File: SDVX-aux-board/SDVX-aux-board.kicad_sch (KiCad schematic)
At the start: 6 parts, among them CN1 AudioJack4_SwitchTR1, CN2 Conn_01x04

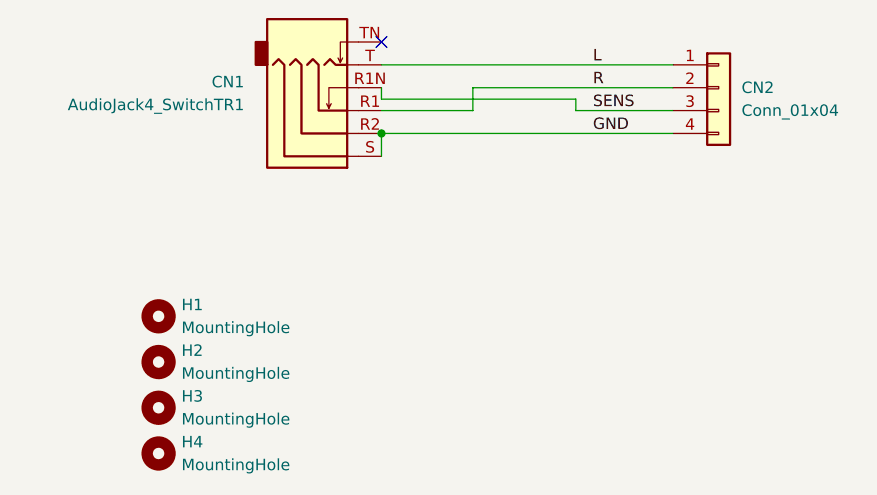
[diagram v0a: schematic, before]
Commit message: Update to working design (kicad 8.0)
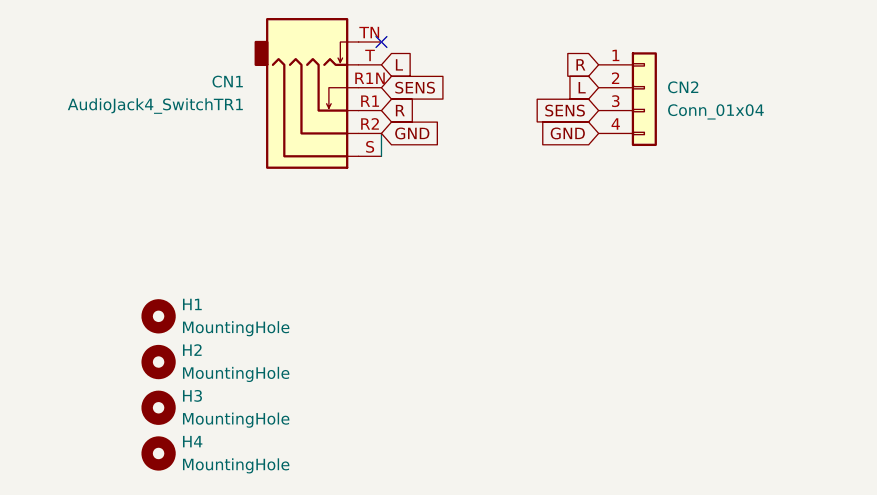
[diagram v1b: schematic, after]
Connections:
- net L: now also CN2.2 (Pin_2); no longer CN2.1 (Pin_1)
- net R: now also CN2.1 (Pin_1); no longer CN2.2 (Pin_2)
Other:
- moved on the sheet: CN2
